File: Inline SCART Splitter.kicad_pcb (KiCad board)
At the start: 2 copper layers, 59 x 49.8 mm, 40 parts, among them J1 SCART-F, J2 USB_B_Micro, J3 SCART-F, J4 SCART-F, U1 THS7374

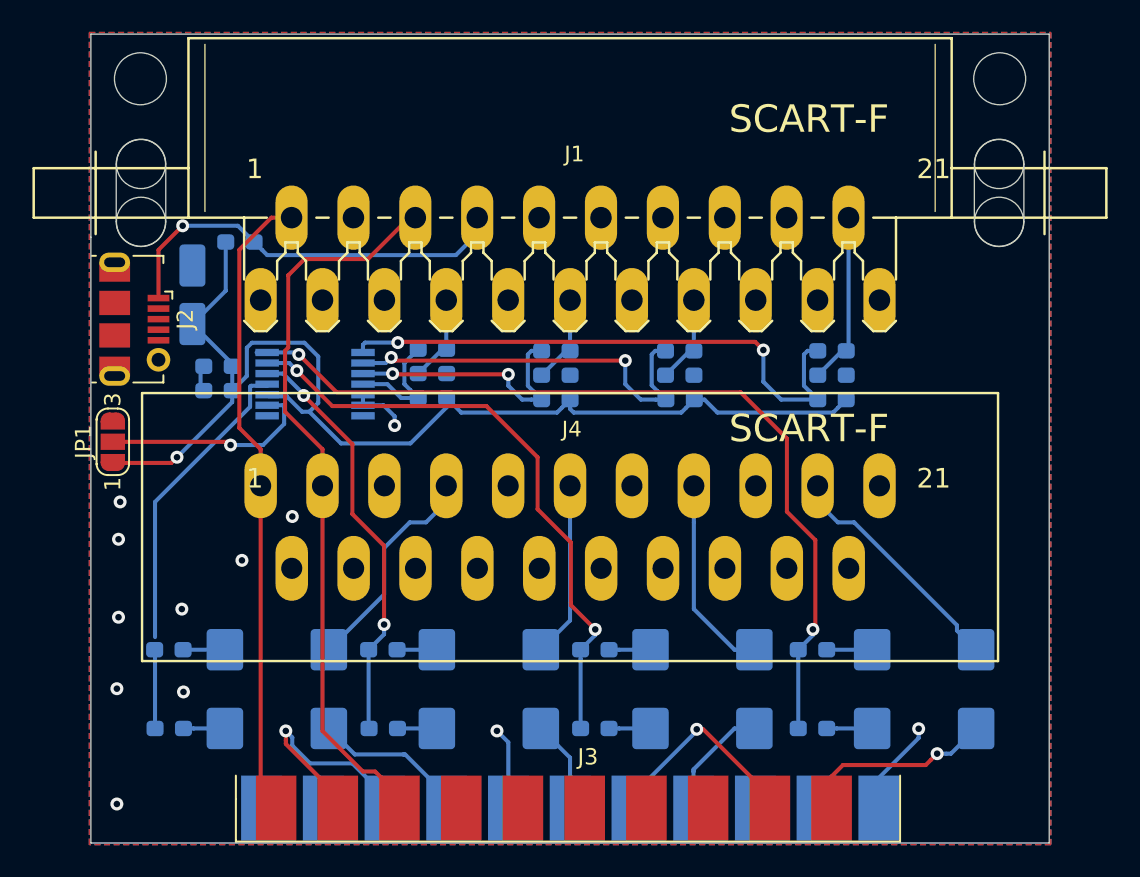
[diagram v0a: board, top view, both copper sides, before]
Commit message: Finished board, added renders
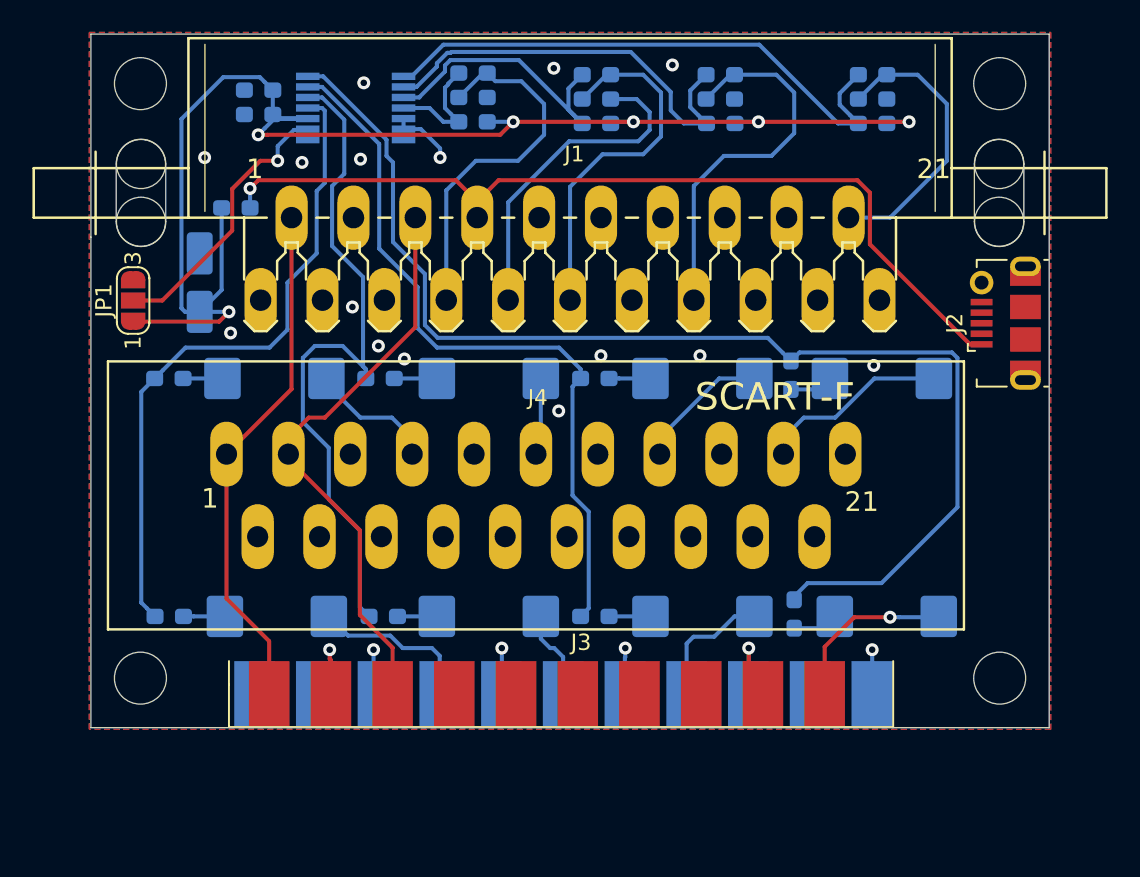
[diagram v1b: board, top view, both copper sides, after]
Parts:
- added REF**: MountingHole_3.2mm_M3, MountingHole:MountingHole_3.2mm_M3, F.Cu at (106.0, 63.1)
- added REF**: MountingHole_3.2mm_M3, MountingHole:MountingHole_3.2mm_M3, F.Cu at (158.9, 63.1)
- moved J2 53.6 mm to (159.3, 41.3), turned to 90 degrees
- moved C1 17.2 mm to (113.3, 28.4)
- moved C2 17.2 mm to (113.3, 26.9)
- moved C4 17.2 mm to (151.1, 26.0)
- moved C5 17.2 mm to (141.8, 26.0)
- moved C6 17.2 mm to (134.1, 26.0)
- moved C7 17.2 mm to (126.5, 25.9)
- moved R1 17.2 mm to (151.1, 27.5)
- moved R2 17.2 mm to (141.8, 27.5)
- moved R3 17.2 mm to (134.1, 27.5)
- moved R4 17.2 mm to (126.5, 27.4)
- moved R5 17.2 mm to (151.1, 29.0)
- moved R6 17.2 mm to (141.8, 29.0)
- moved R7 17.2 mm to (134.1, 29.0)
- moved R8 17.2 mm to (126.5, 28.9)
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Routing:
- net Net-(FB1-Pad2): track 25.5 -> 54.6 mm
- net Net-(R13-Pad2): track 53.9 -> 74.7 mm, vias 2 -> 0
- net RED_IN: track 5.49 -> 23.6 mm
- net BLUE_IN: track 5.40 -> 22.8 mm
- net GREEN_IN: track 5.49 -> 22.5 mm
- net Net-(R12-Pad2): track 23.9 -> 40.3 mm
- net Net-(R11-Pad2): track 25.9 -> 42.3 mm, vias 2 -> 0
- net 5V: track 72.9 -> 88.4 mm, vias 1 -> 6
- net LEFT: track 45.5 -> 35.8 mm
- net Net-(R10-Pad2): track 37.6 -> 45.3 mm, vias 2 -> 0
- net RIGHT: track 39.3 -> 32.0 mm
- net SYNC_IN: track 10.6 -> 17.8 mm
- net Net-(C14-Pad2): track 10.8 -> 4.78 mm
- net Net-(C15-Pad2): track 13.7 -> 7.98 mm
- net Net-(C13-Pad2): track 12.4 -> 8.35 mm
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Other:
- board size 59 x 49.8 mm -> 59 x 42.7 mm
